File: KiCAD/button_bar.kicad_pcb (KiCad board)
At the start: 2 copper layers, 13 parts, among them P1 CONN_4, SW1 SW_UP, SW2 SW_DN, SW3 SW_OK, SW4 SW_LT, SW5 SW_RT, SW6 RESET

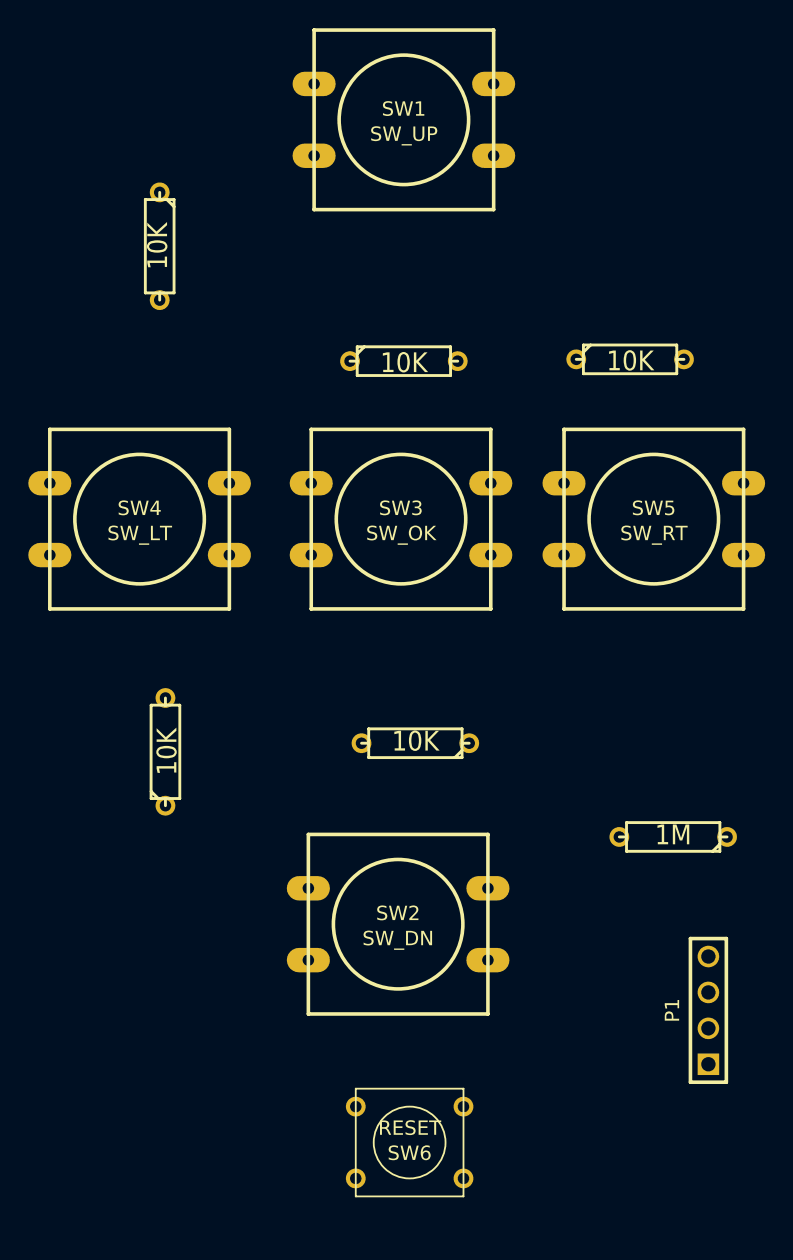
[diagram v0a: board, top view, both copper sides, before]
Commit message: button board schematic update
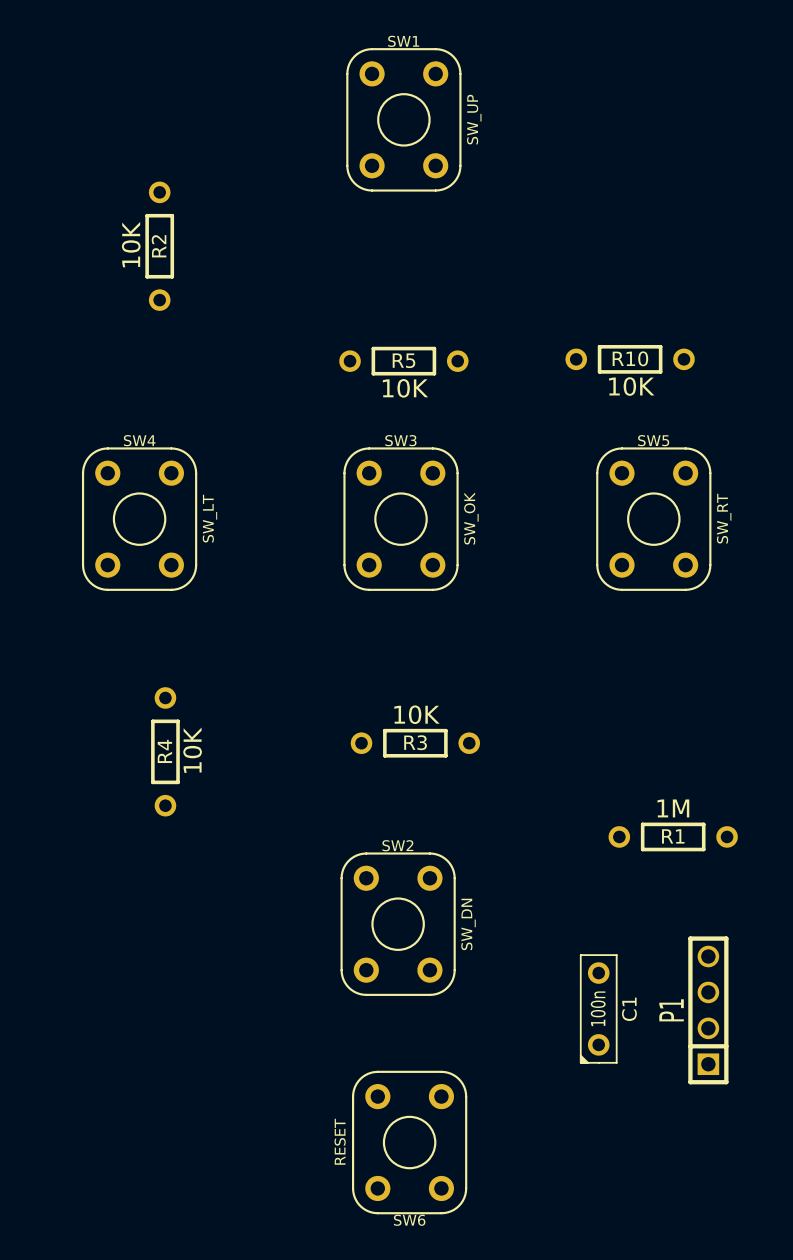
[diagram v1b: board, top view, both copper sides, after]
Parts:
- added C1: 100n, C2, F.Cu at (222.9, 104.8)
- P1: value CONN_4 -> Buttons; footprint PIN_ARRAY_4x1 -> SIL-4
- R1, R10, R2, R3, R4, R5: footprint R3 -> RC03
- SW1, SW2, SW3, SW4, SW5: footprint SW_PUSH-12mm -> SW-PB
- SW6: footprint SW_PUSH_SMALL -> SW-PB
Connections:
- P1 pad 1: N-000001 (its old number) -> /PWR
- P1 pad 4: N-000004 (its old number) -> /RST
- R2 pad 1: N-000001 (its old number) -> /PWR
- SW1 pad 1: N-000001 (its old number) -> /PWR
- SW6 pad 2: N-000004 (its old number) -> /RST
